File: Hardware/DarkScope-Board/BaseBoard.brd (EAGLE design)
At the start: 118.4 x 80 mm, 87 parts, among them IC1 7805DT, IC2 REG1117, IC3 7905, J1 DCJ0202, Q1 8MHz, T2 9014, U1 STM32F103CBT6, X1 TSW-102-07-G-S, X2 TSW-102-07-G-S, X3 MINI-USB-32005-301, X4 2540-5

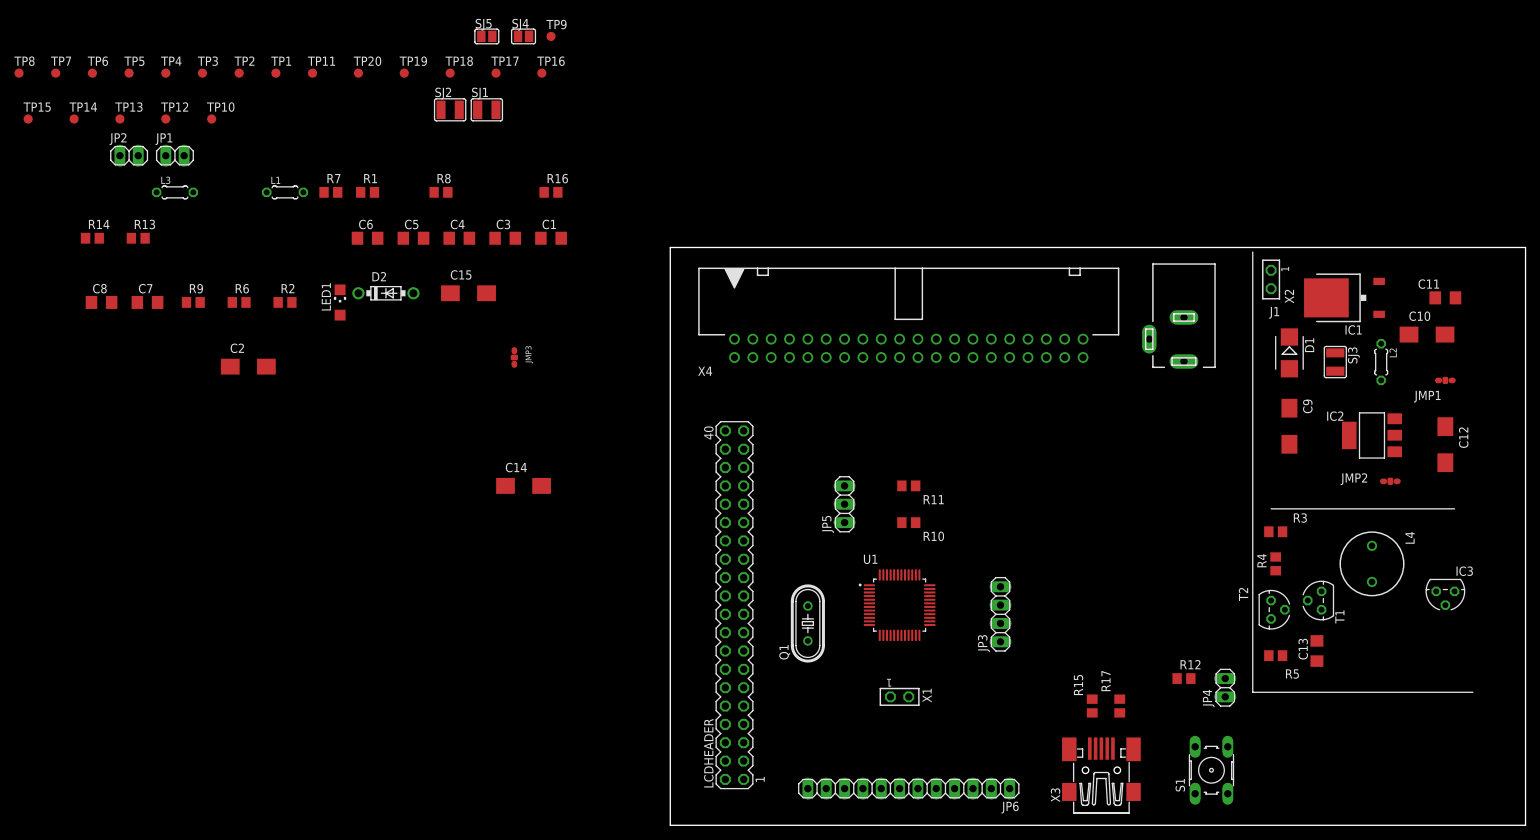
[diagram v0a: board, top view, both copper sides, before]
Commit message: CP Component Placements
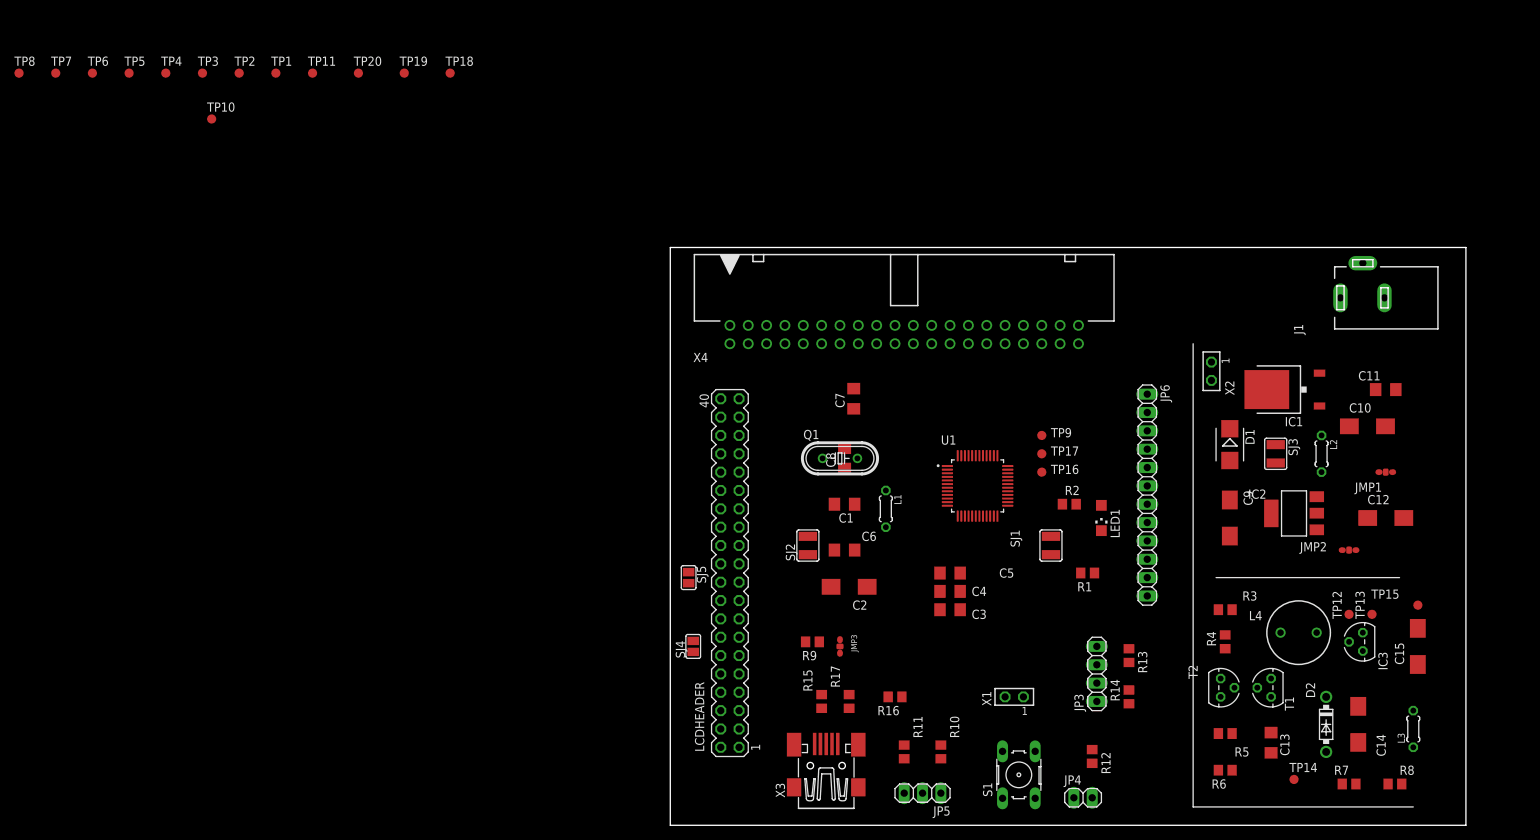
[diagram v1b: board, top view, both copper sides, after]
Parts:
- removed JP1, JP2: (no value), pinhead:1X02
- moved TP15 203.8 mm to (103.5, 30.5), turned to 90 degrees
- moved TP14 192.1 mm to (86.4, 6.35)
- moved L3 186.9 mm to (102.9, 13.3), turned to 90 degrees
- moved TP13 186.4 mm to (97.2, 29.2)
- moved TP12 177.6 mm to (94.0, 29.2), turned to 90 degrees
- moved R7 163.0 mm to (94.0, 5.71), turned to 180 degrees
- moved R14 156.9 mm to (63.5, 17.8), turned to 90 degrees
- moved R8 155.4 mm to (100.3, 5.71)
- moved R6 151.1 mm to (76.8, 7.62)
- moved R13 148.8 mm to (63.5, 23.5), turned to 270 degrees
- moved D2 143.2 mm to (90.8, 14.0), turned to 270 degrees
- moved C15 140.2 mm to (103.5, 24.8), turned to 90 degrees
- moved C14 120.2 mm to (95.2, 14.0), turned to 90 degrees
- moved R1 112.8 mm to (57.8, 34.9), turned to 180 degrees
- moved R2 112.1 mm to (55.2, 44.5)
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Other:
- board size 118.4 x 80 mm -> 110.2 x 80 mm
